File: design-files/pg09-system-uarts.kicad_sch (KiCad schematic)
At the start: 11 parts, among them U701 W65C51, U702 16550, U703 74AHC05, U704 Ali_Express_FTDI_Breakout, U705 Adafruit_FTDI_Friend, X701 1.8432MHz

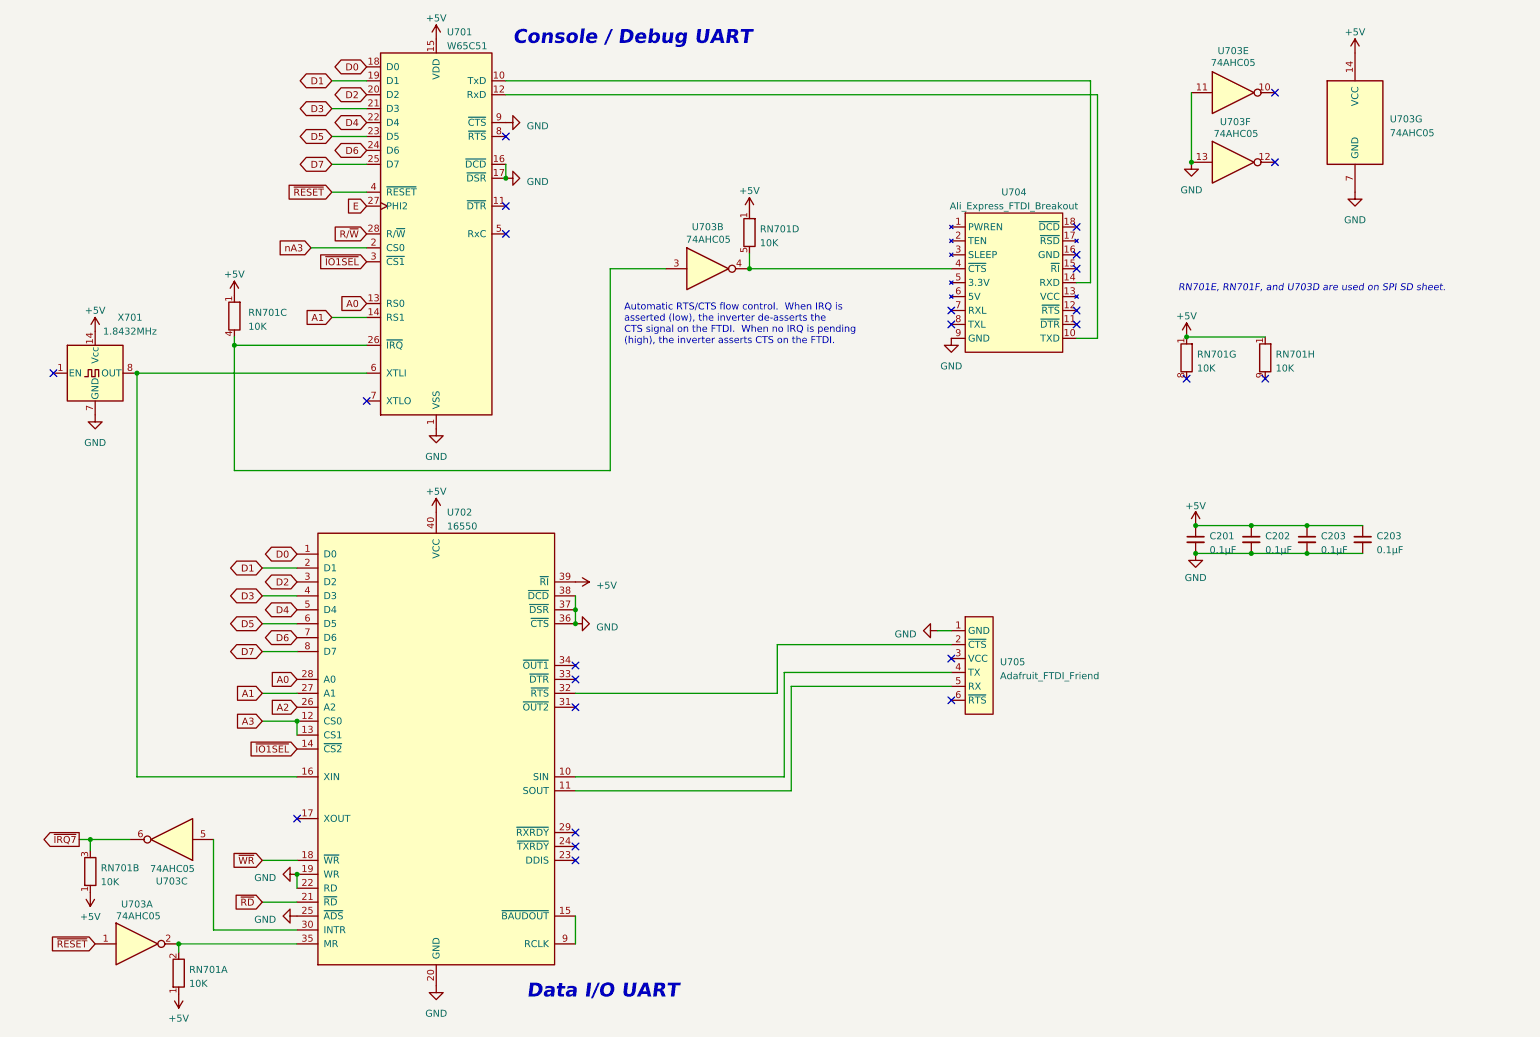
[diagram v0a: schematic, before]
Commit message: Re-do the UARTs using a single TL16C2552 dual-UART in PLCC-44 package.
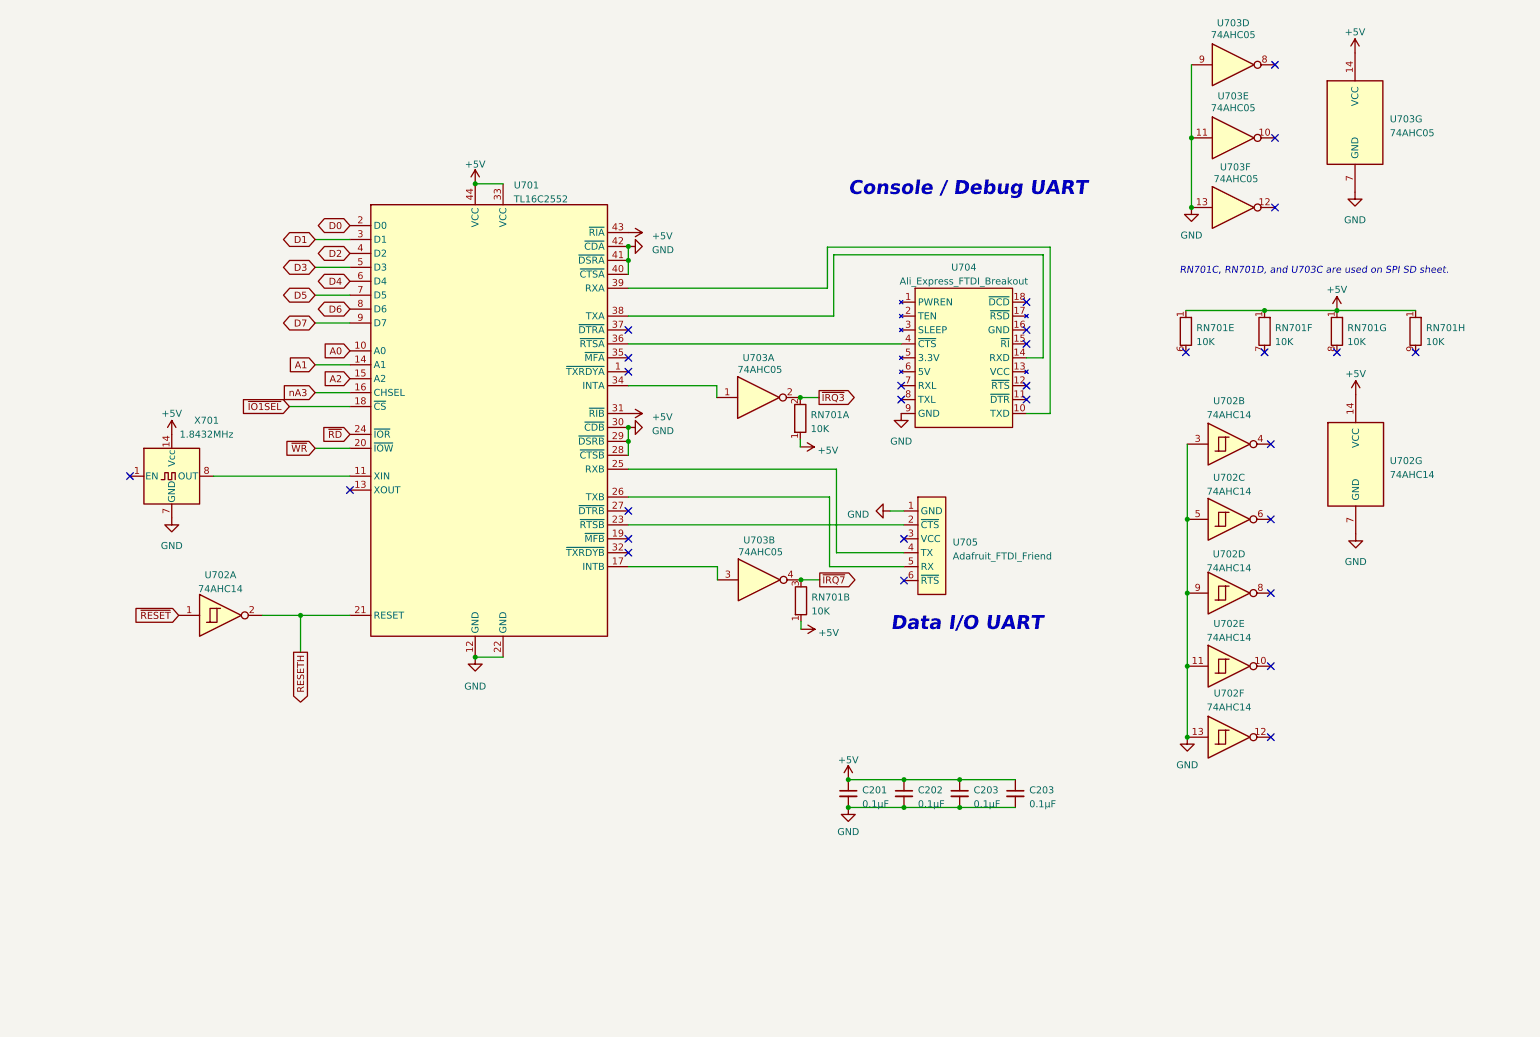
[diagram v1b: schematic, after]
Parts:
- removed unit 3 of RN701
- removed unit 4 of RN701
- removed U701: W65C51, Package_DIP:DIP-28_W15.24mm_Socket, symbol jrt-ICs:W65C51
- removed U702: 16550, Package_DIP:DIP-40_W15.24mm_Socket, symbol Interface_UART:16550
- removed unit 3 of U703
- added unit 5 of RN701
- added unit 6 of RN701
- added U701: TL16C2552, Package_LCC:PLCC-44_THT-Socket, symbol jrt-ICs:TL16C2552
- added U702: 74AHC14, Package_DIP:DIP-14_W7.62mm_Socket, symbol 74xx:74HC14
- added unit 4 of U703
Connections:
- net +5V: now also RN701.1 (R1), RN701.1 (R1), U701.31 (~{RIB}), U701.33 (VCC), U701.43 (~{RIA}), U701.44 (VCC), U702.14 (VCC)
- net A0: now also U701.10 (A0)
- net A1: now also U701.14 (A1)
- net A2: now also U701.15 (A2)
- net D0: now also U701.2 (D0)
- net D1: now also U701.3 (D1)
- net D2: now also U701.4 (D2)
- net D3: now also U701.5 (D3)
- net D4: now also U701.6 (D4)
- net D5: now also U701.7 (D5)
- net D6: now also U701.8 (D6)
- net D7: now also U701.9 (D7)
- net GND: now also U701.12 (GND), U701.22 (GND), U701.28 (~{CTSB}), U701.29 (~{DSRB}), U701.30 (~{CDB}), U701.40 (~{CTSA}), U701.41 (~{DSRA}), U701.42 (~{CDA}), U702.11, U702.13, U702.3, U702.5, U702.7 (GND), U702.9, U703.9
- net nA3: now also U701.16 (CHSEL)
- net ~{IO1SEL}: now also U701.18 (~{CS})
- net ~{IRQ7}: now also U703.4
- net ~{RD}: now also U701.24 (~{IOR})
- net ~{RESET}: now also U702.1; no longer U703.1
- net ~{WR}: now also U701.20 (~{IOW})
- net at U704.10 (TXD): now also U701.39 (RXA)
- net at U704.14 (RXD): now also U701.38 (TXA)
- net at U704.4 (~{CTS}): now also U701.36 (~{RTSA}); no longer U703.4
- net ~{IRQ3}: now reaches RN701.2 (R1.2), U703.2
- net at U703.3: now also U701.17 (INTB)
- net at U705.2 (~{CTS}): now also U701.23 (~{RTSB})
- net at U705.4 (TX): now also U701.25 (RXB)
- net at U705.5 (RX): now also U701.26 (TXB)
- net at X701.8 (OUT): now also U701.11 (XIN)
- new net: U701.34 (INTA), U703.1
- new net RESETH: U701.21 (RESET), U702.2
- no-connect marks 25 -> 29
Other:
- note added: "RN701C, RN701D, and U703C are used on SPI SD sheet."
- note removed: "Automatic RTS/CTS flow control. When IRQ is asserted (low), the inverter de-asserts the CTS signal on the FTDI. When no IRQ is pending (high), the inverter asserts CTS on the FTDI."
- note removed: "RN701E, RN701F, and U703D are used on SPI SD sheet."
- moved on the sheet: C201, C202, C203, RN701A, RN701B, RN701G, RN701H, U703A, U703E, U703F, U704, U705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
